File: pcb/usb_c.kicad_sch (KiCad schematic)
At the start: 6 parts, among them J5 USB_C_Receptacle_USB2.0_14P, U8 TPS2051CDBV, U9 USBLC6-2SC6

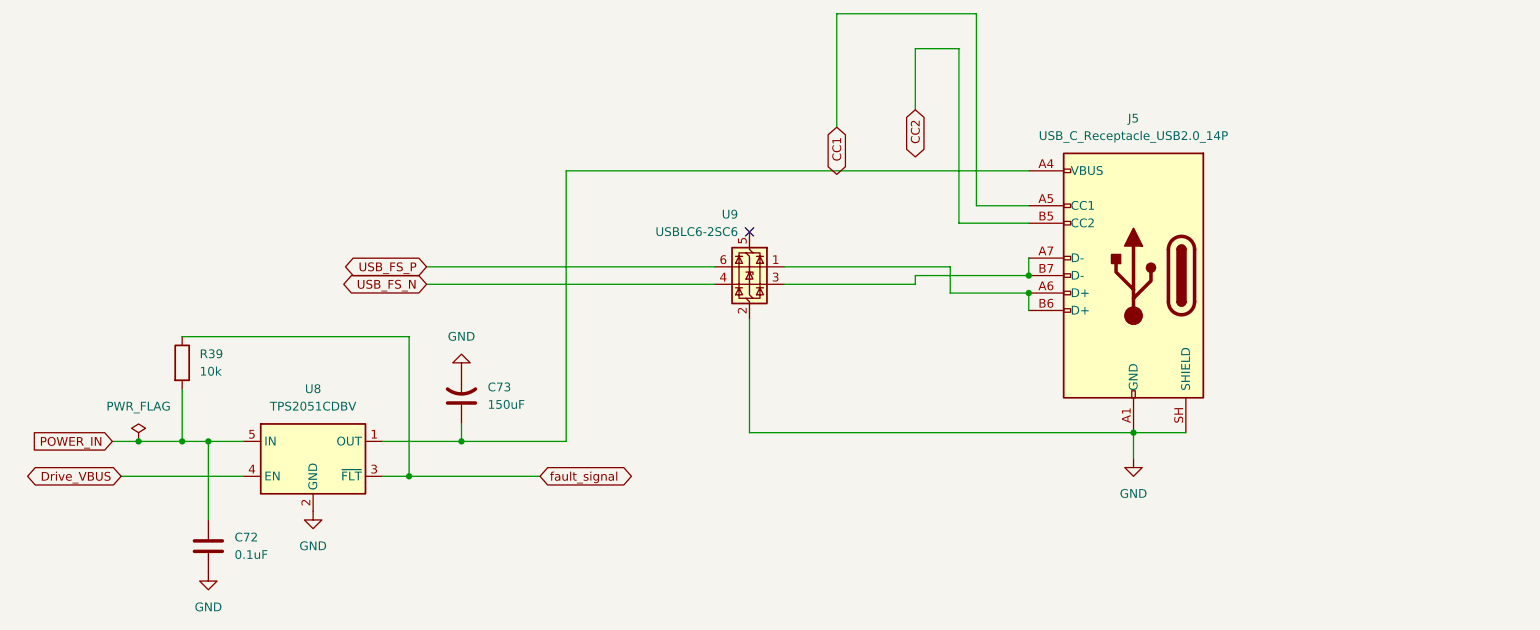
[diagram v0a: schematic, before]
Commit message: layout prep
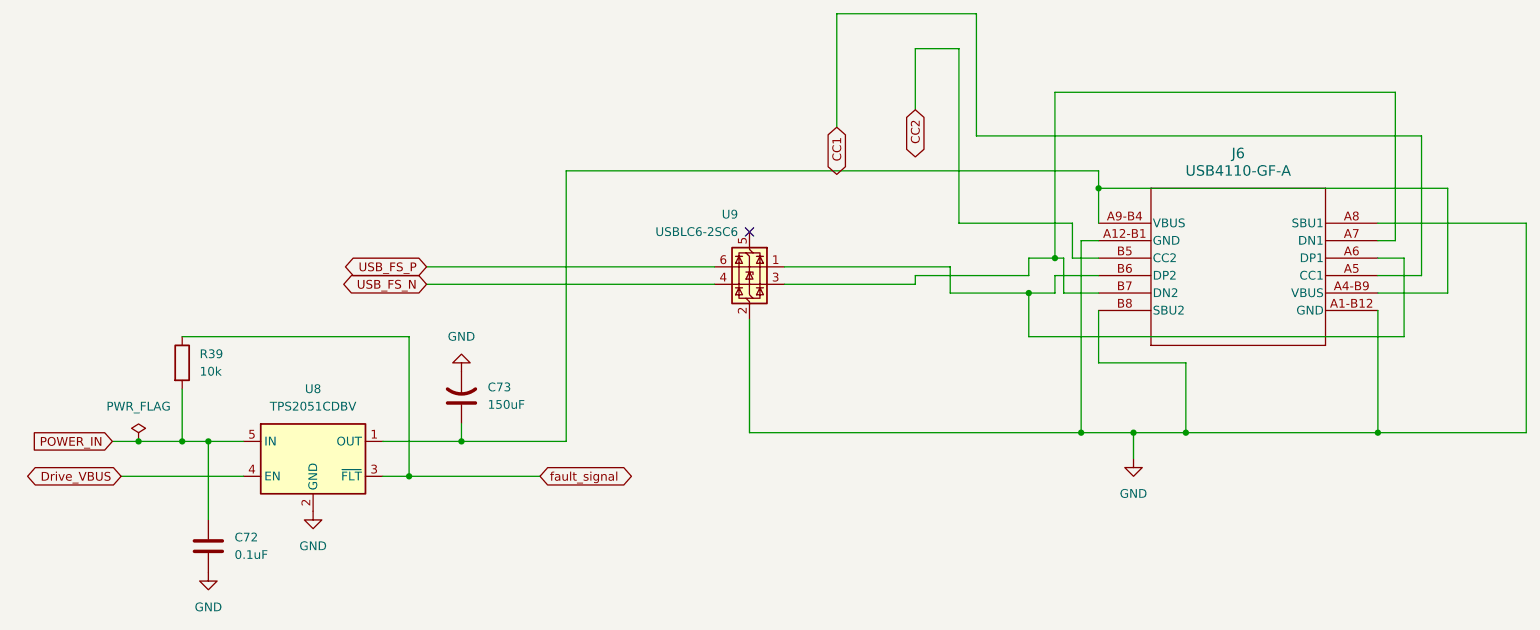
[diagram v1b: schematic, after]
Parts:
- removed J5: USB_C_Receptacle_USB2.0_14P, symbol Connector:USB_C_Receptacle_USB2.0_14P
- added J6: USB4110-GF-A, USB4110_GF_A:USB4110-GF-A_GCT, symbol USB4110_GF_A:USB4110-GF-A
- C72: footprint (none) -> Capacitor_SMD:C_0805_2012Metric_Pad1.18x1.45mm_HandSolder
- C73: footprint Package_TO_SOT_SMD:SOT-23-6 -> Capacitor_SMD:C_0805_2012Metric_Pad1.18x1.45mm_HandSolder
- R39: footprint (none) -> Resistor_SMD:R_0805_2012Metric_Pad1.20x1.40mm_HandSolder
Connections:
- net CC1: now also J6.A5 (CC1)
- net CC2: now also J6.B5 (CC2)
- net GND: now also J6.A1-B12 (GND), J6.A12-B1 (GND), J6.A8 (SBU1), J6.B8 (SBU2)
- net at C73.1, U8.1 (OUT): now also J6.A4-B9 (VBUS), J6.A9-B4 (VBUS)
- net at U9.1 (I/O1): now also J6.A6 (DP1), J6.B6 (DP2)
- net at U9.3 (I/O2): now also J6.A7 (DN1), J6.B7 (DN2)
